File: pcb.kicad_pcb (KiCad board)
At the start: 2 copper layers, 88 x 53 mm, 40 parts, among them J1 TYPE-C-31-M-12, Q1 FDN339AN, SW1 SW_SPST, U1 WeMos_D1_mini, U2 TSOP38236, U3 MCP73831-2-OT, U4 BQ27441DRZR-G1A, U5 TLV75733PDBV

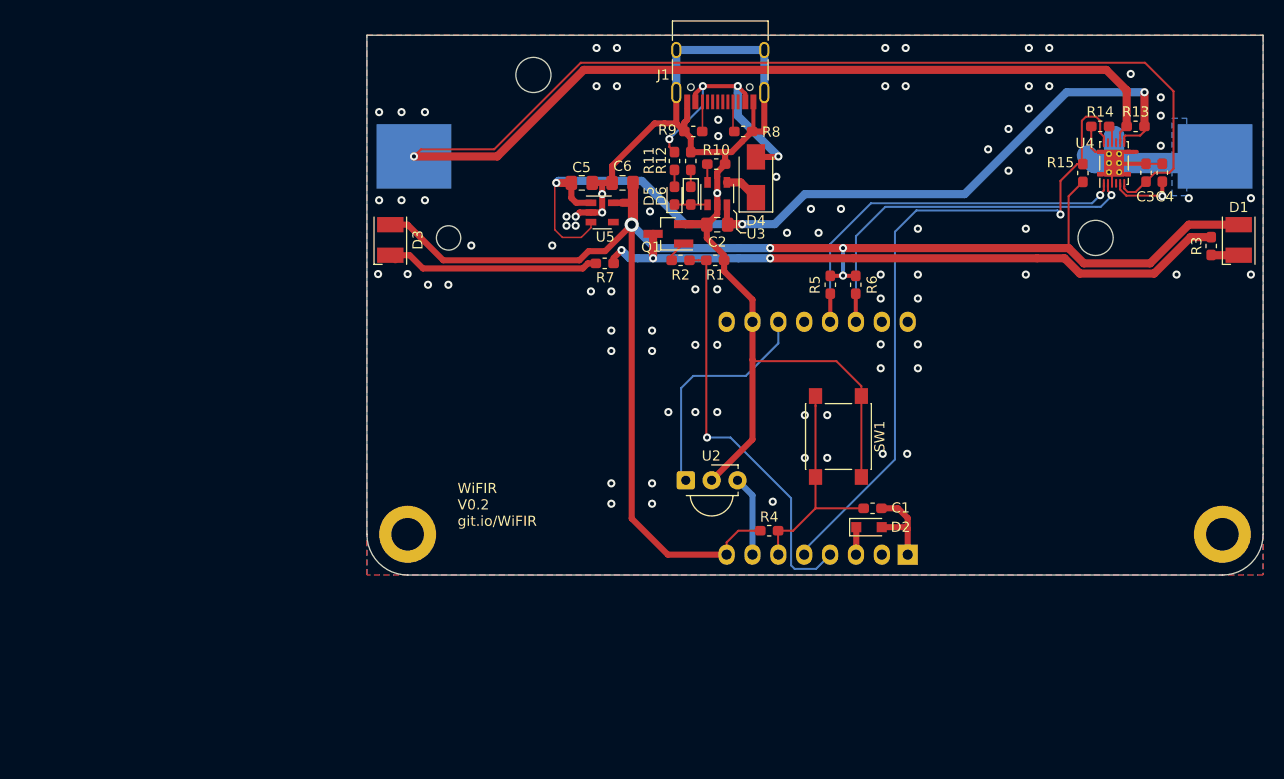
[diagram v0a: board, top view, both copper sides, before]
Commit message: Made it nicer
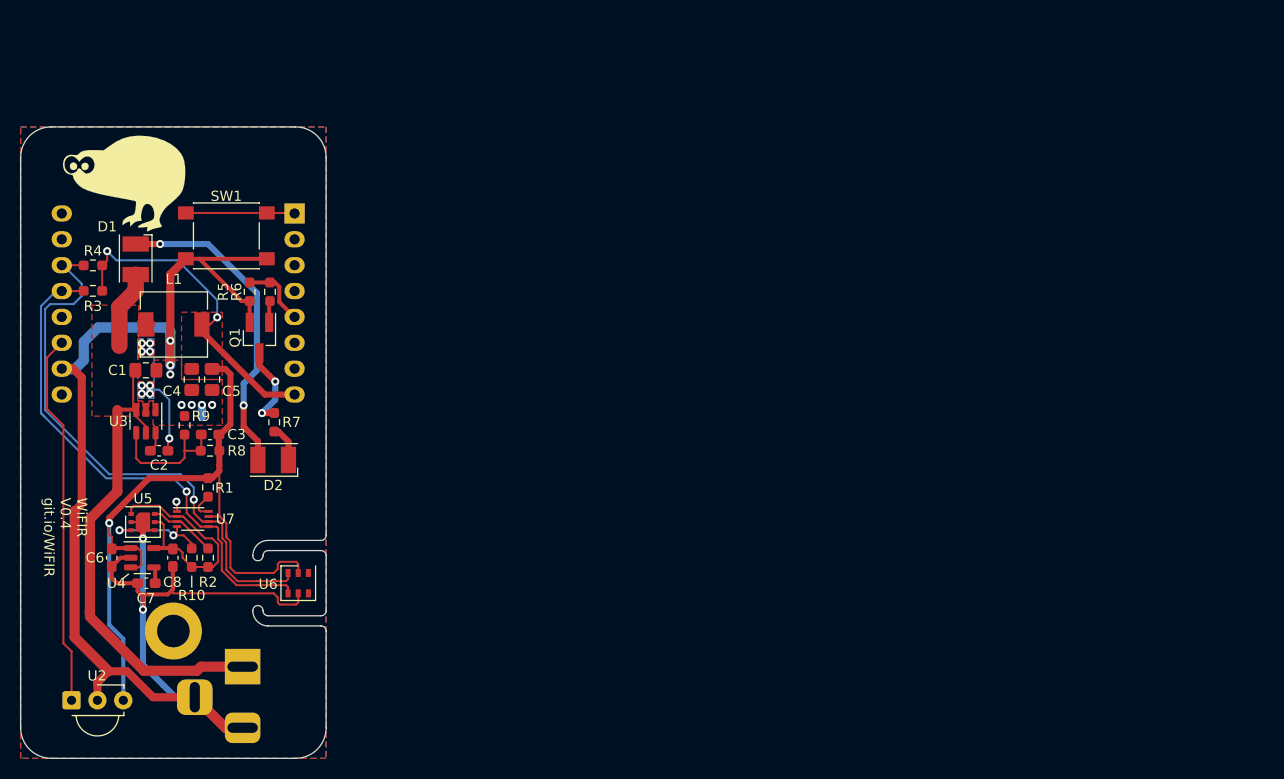
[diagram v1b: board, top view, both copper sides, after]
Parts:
- removed BT1: protected 18650, Battery:BatteryHolder_Keystone_1042_1x18650
- removed D3: VSML3710-GS18, LED_SMD:LED_PLCC-2
- removed D4: MBRA140, Diode_SMD:D_SMA
- removed D5: charging, LED_SMD:LED_0603_1608Metric_Pad1.05x0.95mm_HandSolder
- removed D6: charged, LED_SMD:LED_0603_1608Metric_Pad1.05x0.95mm_HandSolder
- removed the G*** at (189.2, 101.2)
- removed the G*** at (185.2, 101.2)
- removed R11, R12: 470R, Resistor_SMD:R_0603_1608Metric_Pad1.05x0.95mm_HandSolder
- removed R13: 10mR, Resistor_SMD:R_0603_1608Metric_Pad1.05x0.95mm_HandSolder
- removed R14, R15: 10k, Resistor_SMD:R_0603_1608Metric_Pad1.05x0.95mm_HandSolder
- removed the REF** at (178.0, 113.0)
- removed the REF** at (258.0, 113.0)
- added C7: 22nF, Capacitor_SMD:C_0603_1608Metric_Pad1.08x0.95mm_HandSolder, F.Cu at (152.3, 117.8)
- added C8: 1uF, Capacitor_SMD:C_0603_1608Metric_Pad1.08x0.95mm_HandSolder, F.Cu at (154.9, 115.3)
- added G***: LOGO, Graphics:Kiwi-silk, F.Cu at (152.7, 76.7)
- added G***: LOGO, Graphics:Kiwi-silk, B.Cu at (147.9, 116.2)
- added L1: 6.8uH, Inductor_SMD:L_6.3x6.3_H3, F.Cu at (155.1, 92.4)
- added REF**: MountingHole_3.2mm_M3_DIN965_Pad, MountingHole:MountingHole_3.2mm_M3_DIN965_Pad, F.Cu at (155.0, 122.5)
- added U6: AHT20, Package_LGA:Asair_LGA-6_3x3mm_P1mm, F.Cu at (167.3, 117.8)
- added U7: PCA9306DC1, Package_SO:VSSOP-8_2.3x2mm_P0.5mm, F.Cu at (156.9, 111.5)
- C1: value 1uF -> 10uF; footprint Capacitor_SMD:C_0603_1608Metric_Pad1.05x0.95mm_HandSolder -> Capacitor_SMD:C_0805_2012Metric_Pad1.18x1.45mm_HandSolder
- C2: value 4.7uF -> 100nF; footprint Capacitor_SMD:C_0805_2012Metric_Pad1.15x1.40mm_HandSolder -> Capacitor_SMD:C_0603_1608Metric_Pad1.08x0.95mm_HandSolder
- C3: value 10nF -> 47pF; footprint Capacitor_SMD:C_0603_1608Metric_Pad1.05x0.95mm_HandSolder -> Capacitor_SMD:C_0603_1608Metric_Pad1.08x0.95mm_HandSolder
- C4: value 10nF -> 22uF: CL10A226MP8NUNE; footprint Capacitor_SMD:C_0603_1608Metric_Pad1.05x0.95mm_HandSolder -> Capacitor_SMD:C_0805_2012Metric_Pad1.18x1.45mm_HandSolder
- C5: value 4.7uF -> 22uF; footprint Capacitor_SMD:C_0805_2012Metric_Pad1.15x1.40mm_HandSolder -> Capacitor_SMD:C_0805_2012Metric_Pad1.18x1.45mm_HandSolder
- C6: value 4.7uF -> 1uF; footprint Capacitor_SMD:C_0805_2012Metric_Pad1.15x1.40mm_HandSolder -> Capacitor_SMD:C_0603_1608Metric_Pad1.08x0.95mm_HandSolder
- D2: value BAT54WS -> VSML3710-GS18; footprint Diode_SMD:D_SOD-323_HandSoldering -> LED_SMD:LED_PLCC-2
- J1: value TYPE-C-31-M-12 -> 4.5-18V; footprint Connector_USB:USB_C_Receptacle_HRO_TYPE-C-31-M-12 -> Connector_BarrelJack:BarrelJack_Horizontal; moved to B.Cu
- R1: value 4k7 -> 22k; footprint Resistor_SMD:R_0603_1608Metric_Pad1.05x0.95mm_HandSolder -> Resistor_SMD:R_0603_1608Metric_Pad0.98x0.95mm_HandSolder
- R10, R4: value 10k -> 5k1; footprint Resistor_SMD:R_0603_1608Metric_Pad1.05x0.95mm_HandSolder -> Resistor_SMD:R_0603_1608Metric_Pad0.98x0.95mm_HandSolder
- R2: value 1k -> 5k1; footprint Resistor_SMD:R_0603_1608Metric_Pad1.05x0.95mm_HandSolder -> Resistor_SMD:R_0603_1608Metric_Pad0.98x0.95mm_HandSolder
- R3: value 6R8 -> 5k1; footprint Resistor_SMD:R_0603_1608Metric_Pad1.05x0.95mm_HandSolder -> Resistor_SMD:R_0603_1608Metric_Pad0.98x0.95mm_HandSolder
- R5: footprint Resistor_SMD:R_0603_1608Metric_Pad1.05x0.95mm_HandSolder -> Resistor_SMD:R_0603_1608Metric_Pad0.98x0.95mm_HandSolder
- R6: value 4k7 -> 1k; footprint Resistor_SMD:R_0603_1608Metric_Pad1.05x0.95mm_HandSolder -> Resistor_SMD:R_0603_1608Metric_Pad0.98x0.95mm_HandSolder
- R7: value 6R8 -> 27R; footprint Resistor_SMD:R_0603_1608Metric_Pad1.05x0.95mm_HandSolder -> Resistor_SMD:R_0603_1608Metric_Pad0.98x0.95mm_HandSolder
- R8: value 5k1 -> 100k; footprint Resistor_SMD:R_0603_1608Metric_Pad1.05x0.95mm_HandSolder -> Resistor_SMD:R_0603_1608Metric_Pad0.98x0.95mm_HandSolder
- R9: value 5k1 -> 22k; footprint Resistor_SMD:R_0603_1608Metric_Pad1.05x0.95mm_HandSolder -> Resistor_SMD:R_0603_1608Metric_Pad0.98x0.95mm_HandSolder
- U3: value MCP73831-2-OT -> TPS54302; footprint Package_TO_SOT_SMD:SOT-23-5 -> Package_TO_SOT_SMD:SOT-23-6
- U4: value BQ27441DRZR-G1A -> AP131-18; footprint Package_SON:Texas_S-PDSO-N12 -> Package_TO_SOT_SMD:SOT-23-5
- U5: value TLV75733PDBV -> SGP30; footprint Package_TO_SOT_SMD:SOT-23-5 -> Sensor:Sensirion_DFN-6-1EP_2.45x2.45mm_P0.8mm_EP1.25x1.7mm
- moved R3 109.9 mm to (147.1, 89.1), turned to 0 degrees
- moved D1 108.3 mm to (151.3, 86.0), turned to -90 degrees
- moved U4 103.0 mm to (151.9, 115.3), turned to 0 degrees
- moved C4 97.4 mm to (156.8, 97.8), turned to 90 degrees
- moved C3 95.4 mm to (158.6, 103.2), turned to 0 degrees
- moved J1 75.8 mm to (161.8, 126.0), turned to 90 degrees
- moved C1 72.6 mm to (152.3, 96.9), turned to 0 degrees
- moved R4 71.3 mm to (147.1, 86.6), turned to 0 degrees
- moved U1 68.9 mm to (166.9, 81.5), turned to 180 degrees
- moved R10 64.4 mm to (156.8, 115.3), turned to -90 degrees
- moved U2 64.1 mm to (145.0, 129.3)
- moved SW1 63.2 mm to (160.2, 83.7), turned to 180 degrees
- moved C6 62.2 mm to (148.9, 115.3), turned to 90 degrees
- moved R8 61.0 mm to (158.6, 104.8)
- moved U3 60.4 mm to (152.3, 101.9), turned to -90 degrees
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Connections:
- C1 pad 1: ~RST -> VBUS
- C1 pad 2: factory_rst -> GND
- C2 pad 1: GND -> Net-(C2-Pad1)
- C2 pad 2: VCCQ -> Net-(C2-Pad2)
- C3 pad 1: GND -> Net-(C3-Pad1)
- C3 pad 2: +BATT -> +3V3
- C4 pad 2: +1V8 -> +3V3
- C5 pad 1: VCCQ -> GND
- C5 pad 2: GND -> +3V3
- D1 pad 2: +3V3 -> VBUS
- D2 pad 1: device_wake -> Net-(D2-Pad1)
- D2 pad 2: ~RST -> Net-(D1-Pad1)
- R1 pad 1: GND -> Net-(R1-Pad1)
- R1 pad 2: IR_BLAST -> +3V3
- R10 pad 1: GND -> /SDA_1V8
- R10 pad 2: Net-(R10-Pad2) -> +1V8
- R2 pad 1: IR_BLAST -> /SCL_1V8
- R2 pad 2: Net-(Q1-Pad1) -> +1V8
- R3 pad 1: Net-(D1-Pad1) -> /SDA_3V3
- R3 pad 2: Net-(Q1-Pad3) -> +3V3
- R4 pad 1: factory_rst -> /SCL_3V3
- R5 pad 1: SDA -> GND
- R5 pad 2: +3V3 -> IR_BLAST
- R6 pad 1: SCL -> IR_BLAST
- R6 pad 2: +3V3 -> Net-(Q1-Pad1)
- R7 pad 1: Net-(D3-Pad1) -> Net-(D2-Pad1)
- R8 pad 1: Net-(J1-PadA5) -> Net-(C3-Pad1)
- R8 pad 2: GND -> +3V3
- R9 pad 2: Net-(J1-PadB5) -> Net-(C3-Pad1)
- SW1 pad 2: factory_rst -> Net-(SW1-Pad2)
- U1 pad 1: ~RST -> Net-(SW1-Pad2)
- U1 pad 12: Net-(U1-Pad12) -> unconnected-(U1-Pad12)
- U1 pad 13: SDA -> /SDA_3V3
- U1 pad 14: SCL -> /SCL_3V3
- U1 pad 15: Net-(U1-Pad15) -> unconnected-(U1-Pad15)
- U1 pad 16: Net-(U1-Pad16) -> unconnected-(U1-Pad16)
- U1 pad 2: Net-(U1-Pad2) -> unconnected-(U1-Pad2)
- U1 pad 3: device_wake -> unconnected-(U1-Pad3)
- U1 pad 4: IR_BLAST -> unconnected-(U1-Pad4)
- U1 pad 5: ~LOW_BAT -> IR_BLAST
- U1 pad 6: factory_rst -> unconnected-(U1-Pad6)
- U1 pad 7: IR_RECV_VCC -> unconnected-(U1-Pad7)
- U1 pad 9: Net-(U1-Pad9) -> unconnected-(U1-Pad9)
- U2 pad 3: IR_RECV_VCC -> +3V3
- U3 pad 1: Net-(D5-Pad1) -> GND
- U3 pad 2: GND -> Net-(C2-Pad1)
- U3 pad 3: VCCQ -> VBUS
- U3 pad 4: Net-(D4-Pad1) -> Net-(C3-Pad1)
- U3 pad 5: Net-(R10-Pad2) -> VBUS
- U4 pad 1: SDA -> +3V3
- U4 pad 2: SCL -> GND
- U4 pad 3: GND -> +3V3
- U5 pad 1: VCCQ -> +1V8
- U5 pad 3: VCCQ -> /SDA_1V8
- U5 pad 4: Net-(U5-Pad4) -> GND
- U5 pad 5: +3V3 -> +1V8
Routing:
- net +BATT: track 173.7 -> 0.00 mm, vias 1 -> 0
- net VCCQ: track 89.6 -> 0.00 mm, vias 3 -> 0
- net ~LOW_BAT: track 67.6 -> 0.00 mm, vias 1 -> 0
- net Net-(Q1-Pad3): track 64.4 -> 8.29 mm, vias 3 -> 2
- net /SCL_3V3: track 0.00 -> 55.5 mm, vias 0 -> 1
- net /SDA_3V3: track 0.00 -> 51.4 mm, vias 0 -> 1
- net +3V3: track 152.3 -> 105.1 mm, vias 4 -> 3
- net SDA: track 40.3 -> 0.00 mm, vias 1 -> 0
- net SCL: track 39.4 -> 0.00 mm, vias 1 -> 0
- net IR_BLAST: track 41.0 -> 6.72 mm, vias 1 -> 0
- net VBUS: track 26.2 -> 55.5 mm, vias 4 -> 0
- net Net-(D1-Pad1): track 2.71 -> 31.4 mm, vias 0 -> 2
- net factory_rst: track 22.7 -> 0.00 mm
- net Net-(D3-Pad1): track 21.6 -> 0.00 mm
- net +1V8: track 6.53 -> 23.4 mm, vias 1 -> 0
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- added copper zone on F.Cu, net +3V3
- added copper zone on B.Cu, net Net-(C2-Pad1)
- added copper zone on F.Cu, net Net-(C2-Pad1)
- added copper zone on F.Cu, net VBUS
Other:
- board size 88 x 53 mm -> 30 x 62 mm
- net class Default removed
- board text added: "WiFIR V0.4 git.io/WiFIR"
- board text removed: "WiFIR V0.2 git.io/WiFIR"
